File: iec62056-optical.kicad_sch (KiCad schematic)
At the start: 5 parts, among them J1 Conn_01x04_Male, Q1 Q_Photo_NPN

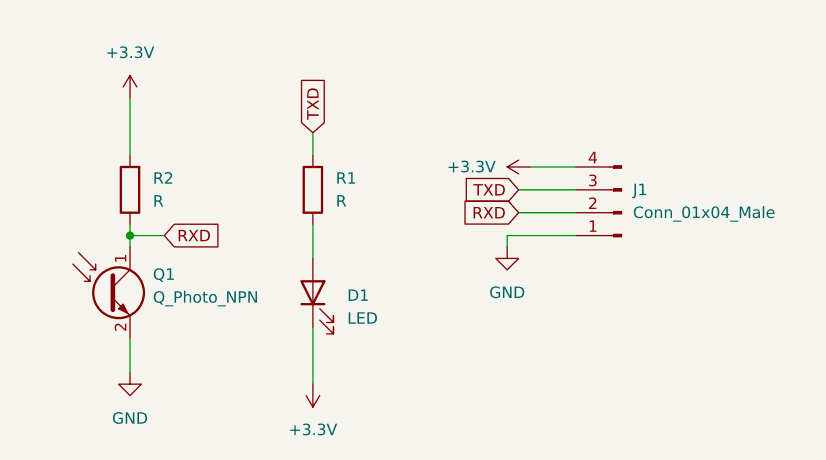
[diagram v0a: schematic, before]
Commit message: version 1.0
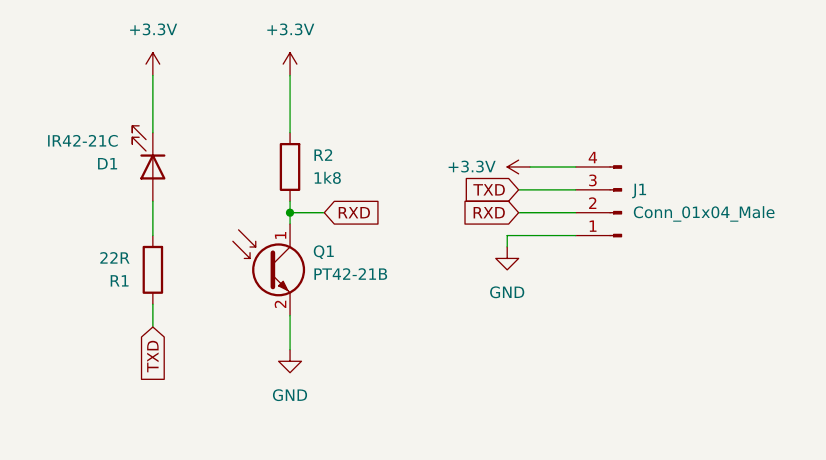
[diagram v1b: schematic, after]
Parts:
- D1: value LED -> IR42-21C; LCSC (none) -> C131198
- Q1: value Q_Photo_NPN -> PT42-21B; LCSC (none) -> C131199
- R1: value R -> 22R; LCSC (none) -> C23345
- R2: value R -> 1k8; LCSC (none) -> C4177
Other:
- moved on the sheet: D1, Q1, R1, R2
